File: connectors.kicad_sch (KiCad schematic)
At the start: 4 parts, among them J1 Conn_01x04_Pin, J2 Conn_01x04_Pin, J3 Conn_01x09_Pin, J4 Conn_02x03_Odd_Even

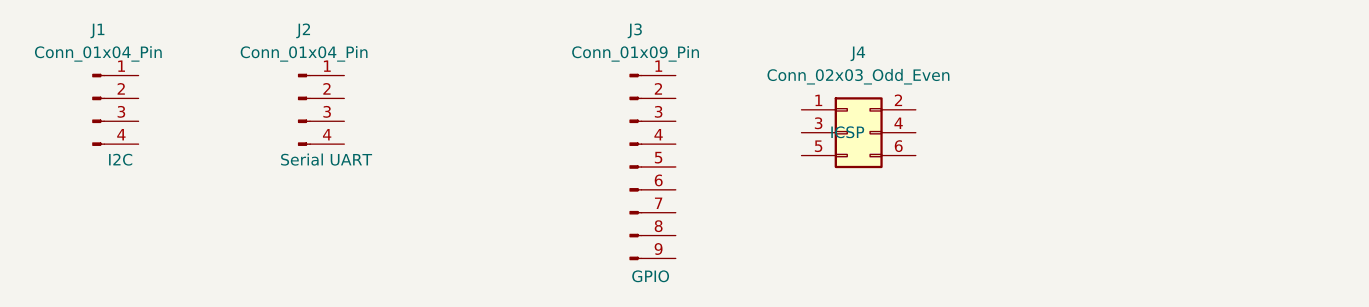
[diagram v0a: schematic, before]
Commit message: finished wiring connector sheet
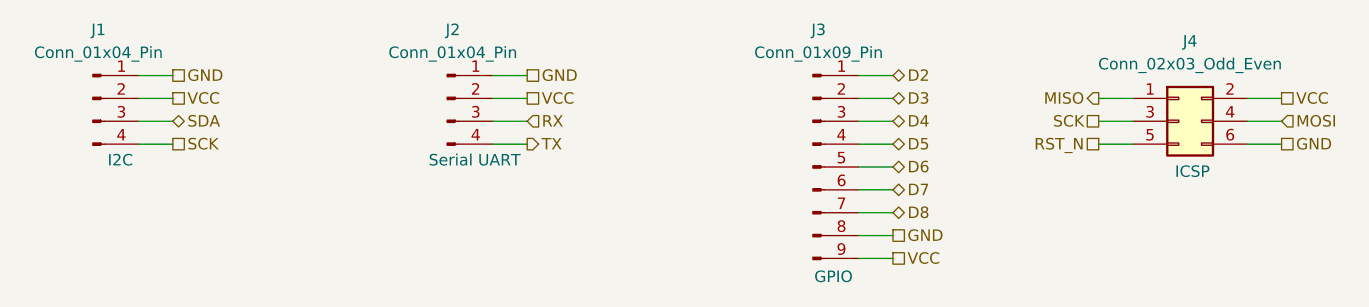
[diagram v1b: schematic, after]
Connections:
- net D2: now reaches J3.1 (Pin_1)
- net D3: now reaches J3.2 (Pin_2)
- net D4: now reaches J3.3 (Pin_3)
- net D5: now reaches J3.4 (Pin_4)
- net D6: now reaches J3.5 (Pin_5)
- net D7: now reaches J3.6 (Pin_6)
- net D8: now reaches J3.7 (Pin_7)
- net GND: now reaches J3.8 (Pin_8)
- net GND: now also J1.1 (Pin_1), J2.1 (Pin_1), J4.6 (Pin_6)
- net VCC: now reaches J3.9 (Pin_9)
- net VCC: now also J1.2 (Pin_2), J2.2 (Pin_2), J4.2 (Pin_2)
- net SDA: now reaches J1.3 (Pin_3)
- net SCK: now reaches J1.4 (Pin_4)
- net SCK: now also J4.3 (Pin_3)
- net RX: now reaches J2.3 (Pin_3)
- net TX: now reaches J2.4 (Pin_4)
- net MISO: now reaches J4.1 (Pin_1)
- net MOSI: now reaches J4.4 (Pin_4)
- net RST_N: now reaches J4.5 (Pin_5)
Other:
- moved on the sheet: J2, J3, J4
